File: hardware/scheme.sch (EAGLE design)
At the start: 30 parts, among them IC1 TINY13-20SSU, Q1 AO3400, Q2 AO3400, Q3 AO3400

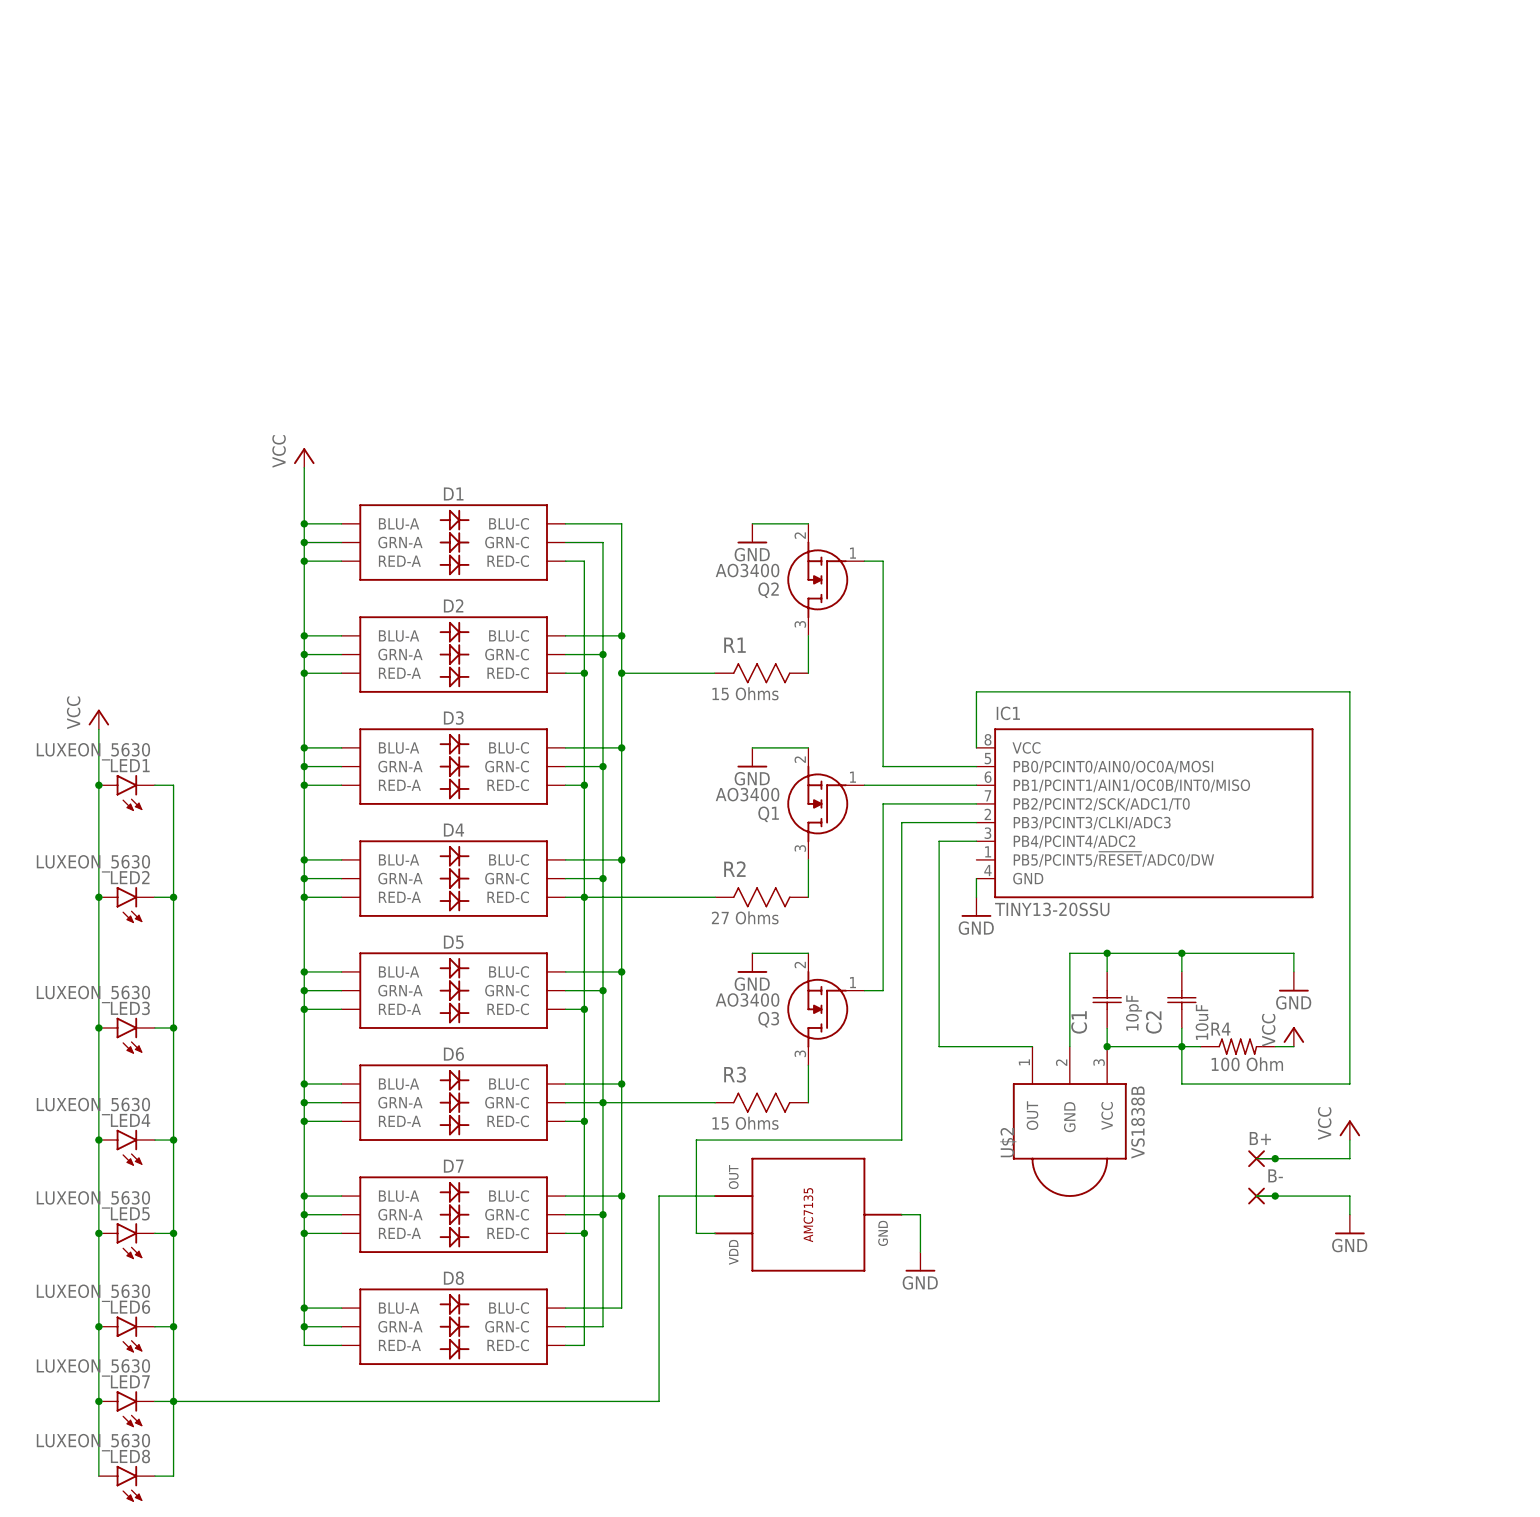
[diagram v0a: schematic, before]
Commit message: RGB version
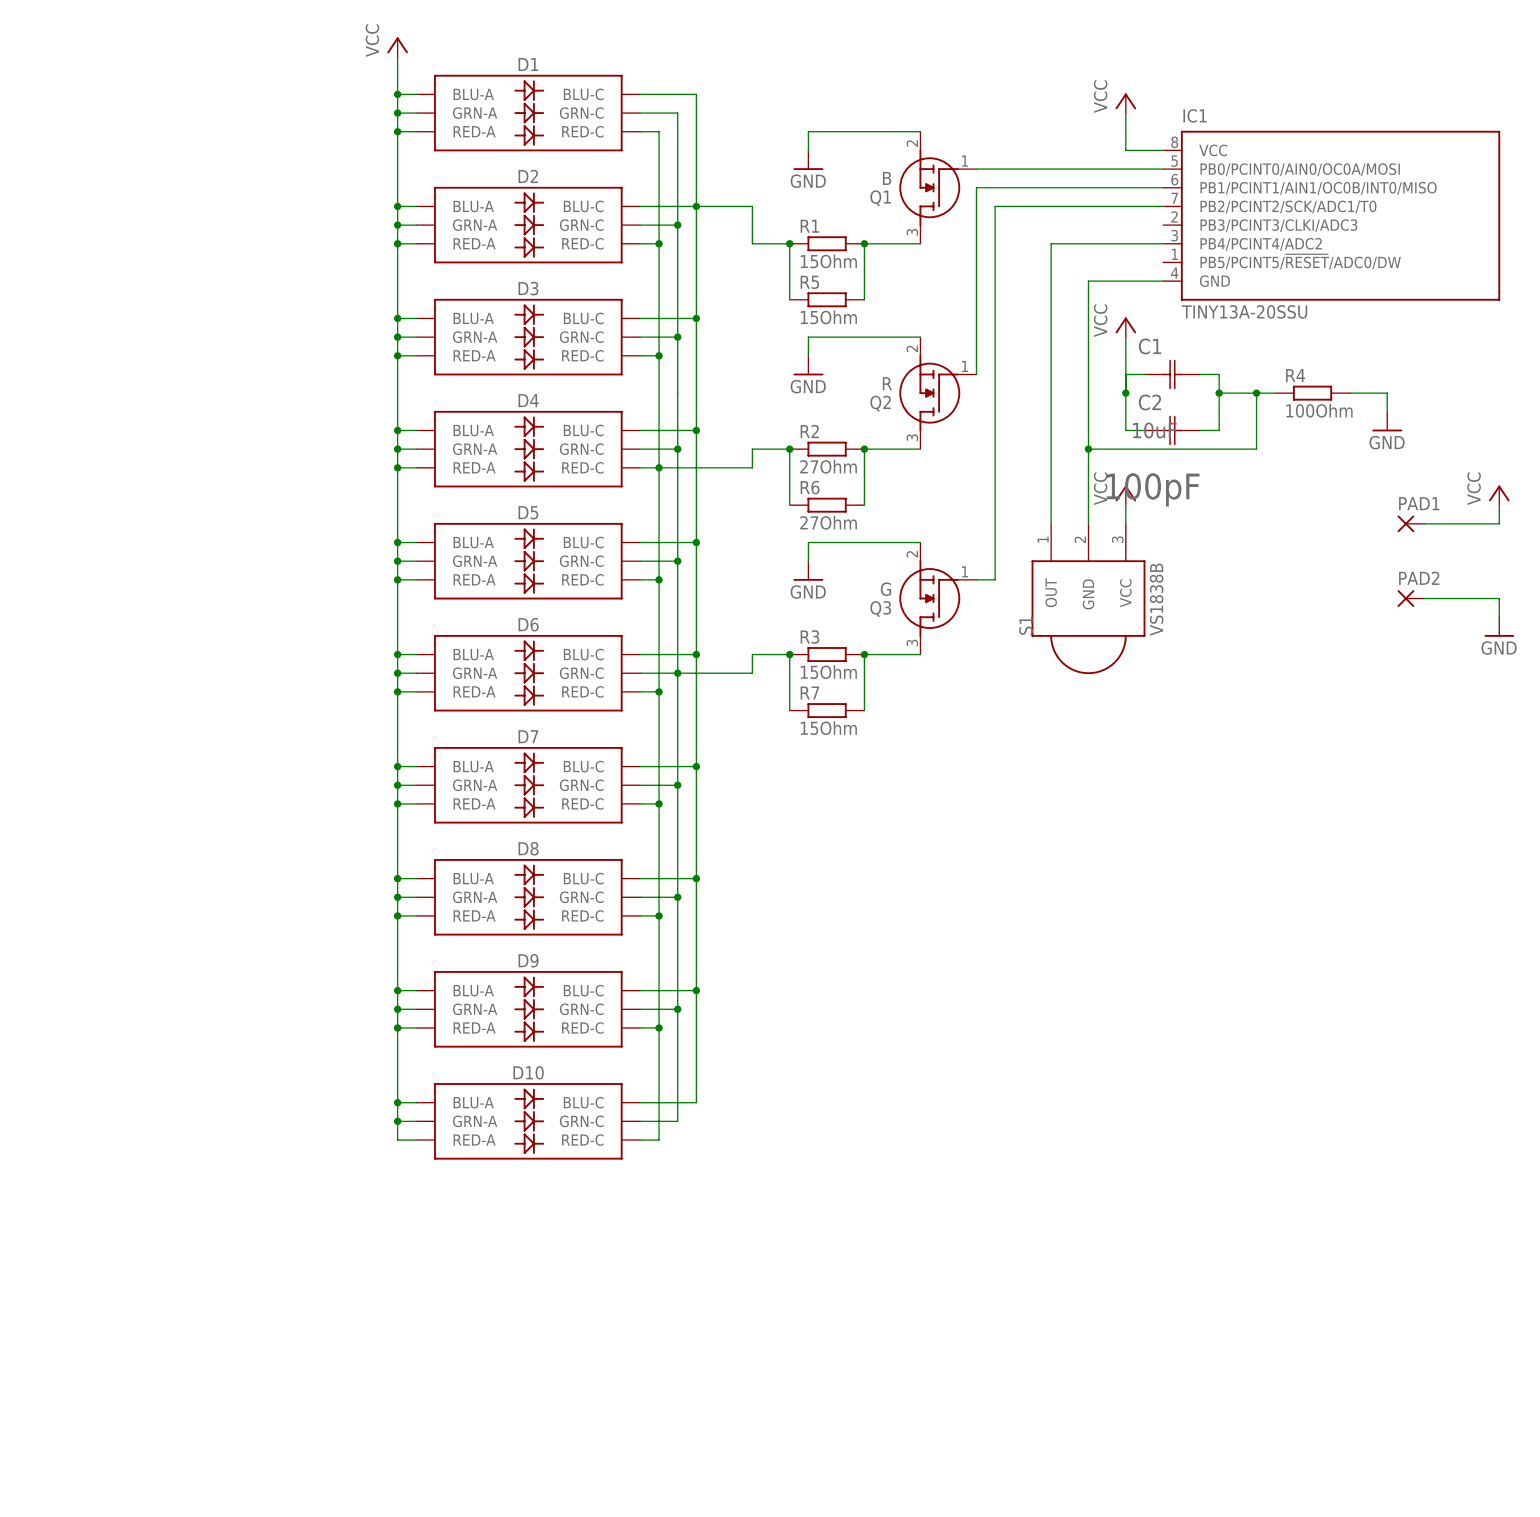
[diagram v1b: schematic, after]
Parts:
- removed B+, B-: WIREPADSMD1,27-254, wirepad:WIREPADSMD1,27-254
- removed LED1, LED2, LED3, LED4, LED5, LED6, LED7, LED8: LUXEON_5630, led:LUXEON_5630
- removed U$1: AMC7135, dan:AMC7135
- removed U$2: VS1838B, adafruit:PNA460XM
- added D10, D9: (no value), 5050_RGB_LED:LED-RGBNO_IC
- added PAD1, PAD2: (no value), wirepad:SMD2
- added R5, R7: 15Ohm, resistor:R-EU_R0805
- added R6: 27Ohm, resistor:R-EU_R0805
- added S1: VS1838B, adafruit:PNA460XM
- C1: value 10pF -> 10uF; device C_0805:08051A100JAT2A -> C_1206:12061A101JAT2A
- C2: value 10uF -> 100pF; device C_1206:12061A101JAT2A -> C_0805:08051A100JAT2A
- D1, D2, D3, D4, D5, D6, D7, D8: device SparkFun-LED:LED-RGBNO_IC -> 5050_RGB_LED:LED-RGBNO_IC
- IC1: value TINY13-20SSU -> TINY13A-20SSU
- Q1: value AO3400 -> B
- Q2: value AO3400 -> R
- Q3: value AO3400 -> G
- R1, R3: value 15 Ohms -> 15Ohm; device R_1206:CRCW1206130RFKEA -> resistor:R-EU_R1206
- R2: value 27 Ohms -> 27Ohm; device R_1206:CRCW1206130RFKEA -> resistor:R-EU_R1206
- R4: value 100 Ohm -> 100Ohm; device rcl:R-US_R0805 -> resistor:R-EU_R0805
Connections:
- removed net N$11: IC1.PB4/PCINT4/ADC2, U$2.OUT
- removed net N$14: C1.C1, C2.C1, IC1.VCC, R4.1, U$2.VCC
- removed net N$5: Q2.D, R1.R1
- new net N$13: D1.RED-C, D10.RED-C, D2.RED-C, D3.RED-C, D4.RED-C, D5.RED-C, D6.RED-C, D7.RED-C, D8.RED-C, D9.RED-C, R2.1, R6.1
- net GND: now also PAD2.P, R4.2; no longer B-.P, C1.C2, C2.C2, IC1.GND, U$1.GND, U$2.GND
- net N$1: now also IC1.PB4/PCINT4/ADC2, S1.OUT; no longer LED1.C, LED2.C, LED3.C, LED4.C, LED5.C, LED6.C, LED7.C, LED8.C, U$1.OUT
- net N$10: now also Q3.D, R3.2, R7.2; no longer D1.BLU-C, D2.BLU-C, D3.BLU-C, D4.BLU-C, D5.BLU-C, D6.BLU-C, D7.BLU-C, D8.BLU-C, R1.R2
- net N$12: now also C1.C2, C2.C2, IC1.GND, R4.1, S1.GND; no longer IC1.PB3/PCINT3/CLKI/ADC3, U$1.VDD
- net N$2: now also Q1.G; no longer Q2.G
- net N$3: now also Q2.G; no longer Q1.G
- net N$6: now also D1.GRN-C, D10.GRN-C, D2.GRN-C, D3.GRN-C, D4.GRN-C, D5.GRN-C, D6.GRN-C, D7.GRN-C, D8.GRN-C, D9.GRN-C, R3.1, R7.1; no longer Q1.D, R2.R1
- net N$7: now also D1.BLU-C, D10.BLU-C, D2.BLU-C, D3.BLU-C, D4.BLU-C, D5.BLU-C, D6.BLU-C, D7.BLU-C, D8.BLU-C, D9.BLU-C, R1.1, R5.1; no longer Q3.D, R3.R1
- net N$8: now also Q1.D, R1.2, R5.2; no longer D1.RED-C, D2.RED-C, D3.RED-C, D4.RED-C, D5.RED-C, D6.RED-C, D7.RED-C, D8.RED-C, R2.R2
- net N$9: now also Q2.D, R2.2, R6.2; no longer D1.GRN-C, D2.GRN-C, D3.GRN-C, D4.GRN-C, D5.GRN-C, D6.GRN-C, D7.GRN-C, D8.GRN-C, R3.R2
- net VCC: now also C1.C1, C2.C1, D10.BLU-A, D10.GRN-A, D10.RED-A, D9.BLU-A, D9.GRN-A, D9.RED-A, IC1.VCC, PAD1.P, S1.VCC; no longer B+.P, LED1.A, LED2.A, LED3.A, LED4.A, LED5.A, LED6.A, LED7.A, LED8.A, R4.2
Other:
- moved on the sheet: C1, C2, D1, D2, D3, D4, D5, D6, D7, D8, IC1, Q1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
